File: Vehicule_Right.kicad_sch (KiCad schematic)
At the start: 16 parts, among them Q27 IRLZ44N, U7 LM339

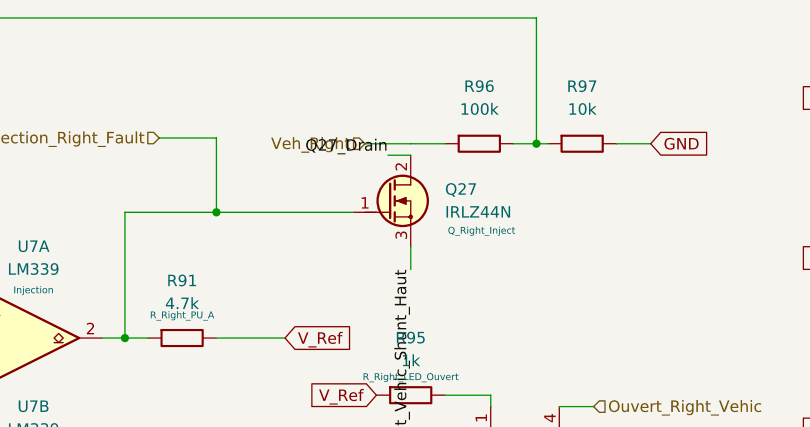
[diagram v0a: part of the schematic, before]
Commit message: Add files via upload
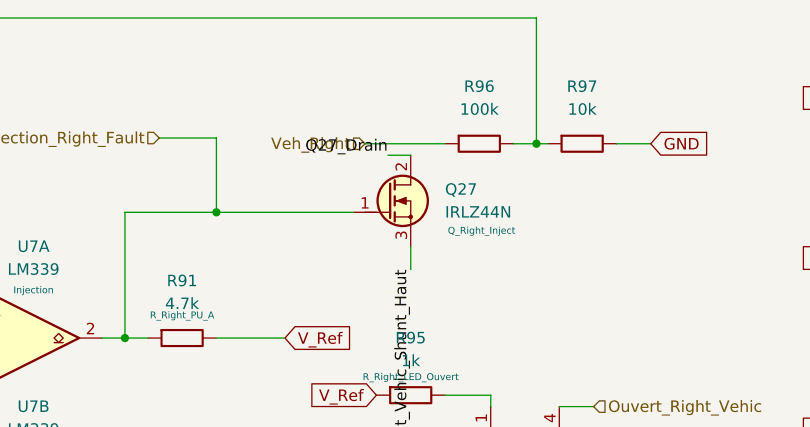
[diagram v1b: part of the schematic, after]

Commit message: Add files via upload
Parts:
- U7: footprint (none) -> Package_DIP:DIP-14_W7.62mm_Socket
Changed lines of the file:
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@@
 			)
 		)
-		(property "Footprint" ""
+		(property "Footprint" "Package_DIP:DIP-14_W7.62mm_Socket"
 			(at 110.49 134.62 0)
 			(hide yes)
@@
 			)
 		)
-		(property "Footprint" ""
+		(property "Footprint" "Package_DIP:DIP-14_W7.62mm_Socket"
 			(at 113.03 116.84 0)
 			(hide yes)
@@
 			)
 		)
-		(property "Footprint" ""
+		(property "Footprint" "Package_DIP:DIP-14_W7.62mm_Socket"
 			(at 113.03 85.09 0)
 			(hide yes)
@@
 			)
 		)
-		(property "Footprint" ""
+		(property "Footprint" "Package_DIP:DIP-14_W7.62mm_Socket"
 			(at 113.03 101.6 0)
 			(hide yes)
@@
 			)
 		)
-		(property "Footprint" ""
+		(property "Footprint" "Package_DIP:DIP-14_W7.62mm_Socket"
 			(at 113.03 67.31 0)
 			(hide yes)

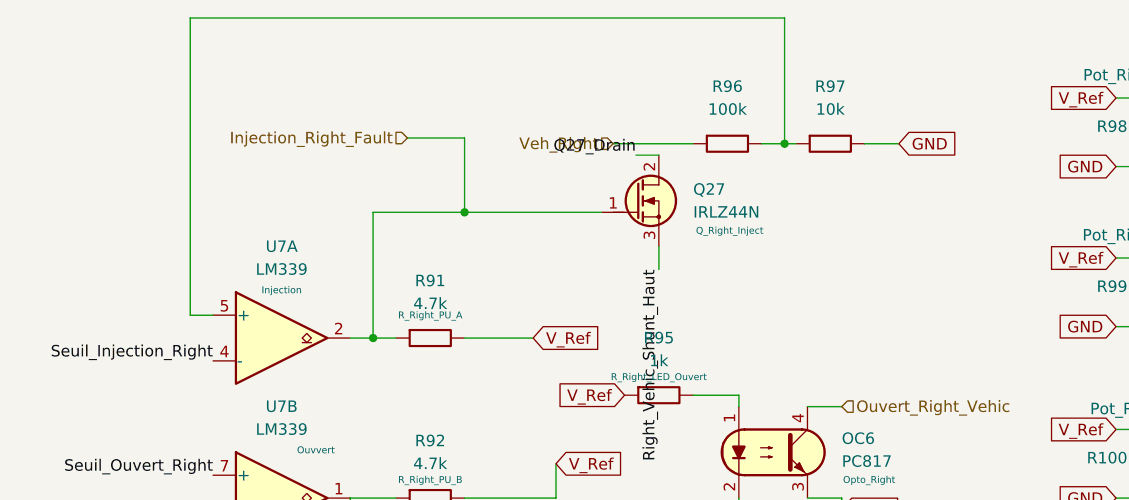
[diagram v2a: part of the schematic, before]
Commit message: Add files via upload
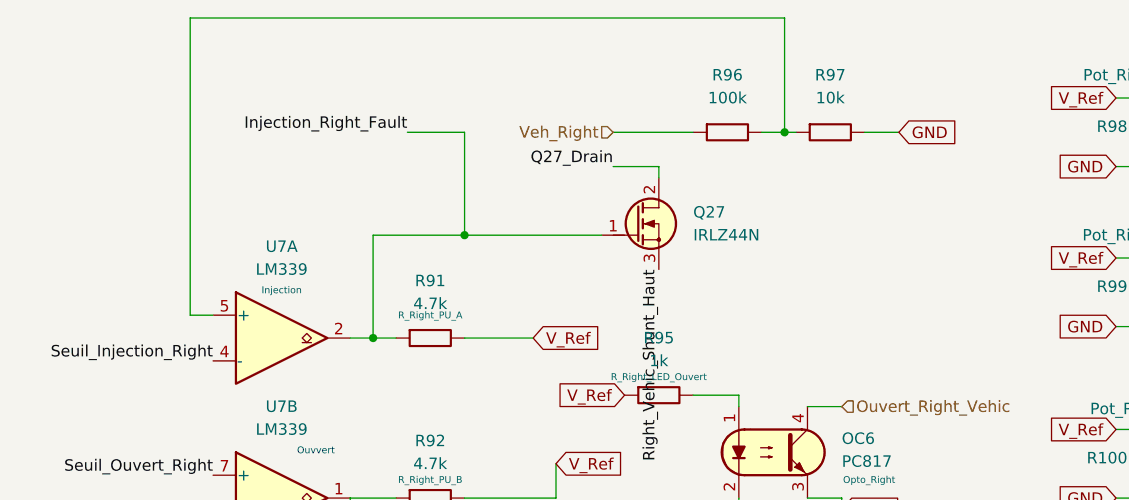
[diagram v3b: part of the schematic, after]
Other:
- moved on the sheet: Q27, R96, R97
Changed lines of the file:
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@@
 	)
 	(junction
-		(at 170.18 48.26)
+		(at 170.18 46.99)
 		(diameter 0)
 		(color 0 0 0 0)
 	)
 	(junction
-		(at 134.62 55.88)
+		(at 124.46 69.85)
 		(diameter 0)
 		(color 0 0 0 0)
 	)
 	(junction
-		(at 124.46 69.85)
+		(at 134.62 58.42)
 		(diameter 0)
 		(color 0 0 0 0)
@@
 	(wire
 		(pts
-			(xy 134.62 55.88) (xy 149.86 55.88)
+			(xy 134.62 58.42) (xy 149.86 58.42)
 		)
 		(stroke
@@
 	(wire
 		(pts
-			(xy 124.46 69.85) (xy 121.92 69.85)
+			(xy 156.21 50.8) (xy 156.21 52.07)
 		)
 		(stroke
@@
 	(wire
 		(pts
-			(xy 156.21 59.69) (xy 156.21 62.23)
+			(xy 124.46 69.85) (xy 121.92 69.85)
 		)
 		(stroke
@@
 	(wire
 		(pts
-			(xy 156.21 49.53) (xy 153.67 49.53)
-		)
-		(stroke
-			(width 0)
-			(type default)
-		)
-	)
-	(wire
-		(pts
 			(xy 207.01 68.58) (xy 210.82 68.58)
 		)
@@
 	(wire
 		(pts
-			(xy 170.18 48.26) (xy 170.18 34.29)
+			(xy 170.18 46.99) (xy 170.18 34.29)
 		)
 		(stroke
@@
 	(wire
 		(pts
-			(xy 170.18 48.26) (xy 171.45 48.26)
+			(xy 170.18 46.99) (xy 171.45 46.99)
 		)
 		(stroke
@@
 	(wire
 		(pts
-			(xy 179.07 48.26) (xy 182.88 48.26)
+			(xy 179.07 46.99) (xy 182.88 46.99)
 		)
 		(stroke
@@
 	(wire
 		(pts
-			(xy 134.62 47.625) (xy 134.62 55.88)
+			(xy 207.01 87.63) (xy 210.82 87.63)
 		)
 		(stroke
@@
 	(wire
 		(pts
-			(xy 207.01 87.63) (xy 210.82 87.63)
+			(xy 170.18 34.29) (xy 104.14 34.29)
 		)
 		(stroke
@@
 	(wire
 		(pts
-			(xy 170.18 34.29) (xy 104.14 34.29)
+			(xy 124.46 58.42) (xy 134.62 58.42)
 		)
 		(stroke
@@
 	(wire
 		(pts
-			(xy 124.46 55.88) (xy 134.62 55.88)
+			(xy 82.55 90.17) (xy 82.55 101.6)
 		)
 		(stroke
@@
 	(wire
 		(pts
-			(xy 82.55 90.17) (xy 82.55 101.6)
+			(xy 140.97 104.14) (xy 140.97 109.22)
 		)
 		(stroke
@@
 	(wire
 		(pts
-			(xy 140.97 104.14) (xy 140.97 109.22)
+			(xy 69.85 132.08) (xy 67.31 132.08)
 		)
 		(stroke
@@
 	(wire
 		(pts
-			(xy 69.85 132.08) (xy 67.31 132.08)
+			(xy 207.01 43.18) (xy 210.82 43.18)
 		)
 		(stroke
@@
 	(wire
 		(pts
-			(xy 207.01 43.18) (xy 210.82 43.18)
+			(xy 134.62 46.99) (xy 134.62 58.42)
 		)
 		(stroke
@@
 	(wire
 		(pts
-			(xy 151.13 48.26) (xy 160.02 48.26)
+			(xy 151.13 46.99) (xy 160.02 46.99)
 		)
 		(stroke
@@
 	(wire
 		(pts
-			(xy 128.27 47.625) (xy 134.62 47.625)
+			(xy 128.27 46.99) (xy 134.62 46.99)
 		)
 		(stroke
@@
 	(wire
 		(pts
-			(xy 167.64 48.26) (xy 170.18 48.26)
+			(xy 167.64 46.99) (xy 170.18 46.99)
 		)
 		(stroke
@@
 	(wire
 		(pts
-			(xy 124.46 55.88) (xy 124.46 69.85)
+			(xy 124.46 58.42) (xy 124.46 69.85)
 		)
 		(stroke
@@
 	(wire
 		(pts
+			(xy 151.13 50.8) (xy 156.21 50.8)
+		)
+		(stroke
+			(width 0)
+			(type default)
+		)
+	)
+	(wire
+		(pts
 			(xy 127 69.85) (xy 124.46 69.85)
 		)
@@
 		)
 	)
+	(label "Injection_Right_Fault"
+		(at 128.27 46.99 180)
+		(effects
+			(font
+				(size 1.27 1.27)
+			)
+			(justify right bottom)
+		)
+	)
 	(label "Seuil_Court_Right"
 		(at 214.63 83.82 0)
@@
 	)
 	(label "Q27_Drain"
-		(at 153.67 49.53 180)
+		(at 151.13 50.8 180)
 		(effects
 			(font
@@
 	(global_label "GND"
 		(shape input)
-		(at 182.88 48.26 0)
+		(at 182.88 46.99 0)
 		(fields_autoplaced yes)
 		(effects
@@
 		)
 		(property "Intersheetrefs" "${INTERSHEET_REFS}"
-			(at 189.7357 48.26 0)
+			(at 189.7357 46.99 0)
 			(hide yes)
 			(show_name no)
@@
 		)
 	)
-	(hierarchical_label "Injection_Right_Fault"
-		(shape input)
-		(at 128.27 47.625 180)
-		(effects
-			(font
-				(size 1.27 1.27)
-			)
-			(justify right)
-		)
-	)
 	(hierarchical_label "Veh_Right"
 		(shape input)
-		(at 151.13 48.26 180)
+		(at 151.13 46.99 180)
 		(effects
 			(font
@@
 	(symbol
 		(lib_id "PCM_SL_Resistors:100k")
-		(at 163.83 48.26 0)
+		(at 163.83 46.99 0)
 		(unit 1)
 		(body_style 1)
@@
 		(fields_autoplaced yes)
 		(property "Reference" "R96"
-			(at 163.83 41.91 0)
+			(at 163.83 40.64 0)
 			(show_name no)
 			(do_not_autoplace no)
@@
 		)
 		(property "Value" "100k"
-			(at 163.83 44.45 0)
+			(at 163.83 43.18 0)
 			(show_name no)
 			(do_not_autoplace no)
@@
 		)
 		(property "Footprint" "Resistor_THT:R_Axial_DIN0207_L6.3mm_D2.5mm_P10.16mm_Horizontal"
-			(at 164.719 52.578 0)
+			(at 164.719 51.308 0)
 			(hide yes)
 			(show_name no)
@@
 		)
 		(property "Datasheet" ""
-			(at 164.338 48.26 0)
+			(at 164.338 46.99 0)
 			(hide yes)
 			(show_name no)
@@
 		)
 		(property "Description" "100kΩ, 1/4W Resistor"
-			(at 163.83 48.26 0)
+			(at 163.83 46.99 0)
 			(hide yes)
 			(show_name no)
@@
 	(symbol
 		(lib_id "PCM_SL_Resistors:10k")
-		(at 175.26 48.26 0)
+		(at 175.26 46.99 0)
 		(unit 1)
 		(body_style 1)
@@
 		(fields_autoplaced yes)
 		(property "Reference" "R97"
-			(at 175.26 41.91 0)
+			(at 175.26 40.64 0)
 			(show_name no)
 			(do_not_autoplace no)
@@
 		)
 		(property "Value" "10k"
-			(at 175.26 44.45 0)
+			(at 175.26 43.18 0)
 			(show_name no)
 			(do_not_autoplace no)
@@
 		)
 		(property "Footprint" "Resistor_THT:R_Axial_DIN0207_L6.3mm_D2.5mm_P10.16mm_Horizontal"
-			(at 176.149 52.578 0)
+			(at 176.149 51.308 0)
 			(hide yes)
 			(show_name no)
@@
 		)
 		(property "Datasheet" ""
-			(at 175.768 48.26 0)
+			(at 175.768 46.99 0)
 			(hide yes)
 			(show_name no)
@@
 		)
 		(property "Description" "10kΩ, 1/4W Resistor"
-			(at 175.26 48.26 0)
+			(at 175.26 46.99 0)
 			(hide yes)
 			(show_name no)
@@
 	(symbol
 		(lib_id "PCM_Transistor_MOSFET_AKL:IRLZ44N")
-		(at 153.67 54.61 0)
+		(at 153.67 57.15 0)
 		(unit 1)
 		(body_style 1)
@@
 		(dnp no)
 		(property "Reference" "Q27"
-			(at 160.02 53.3399 0)
+			(at 160.02 55.8799 0)
 			(show_name no)
 			(do_not_autoplace no)
@@
 		)
 		(property "Value" "IRLZ44N"
-			(at 160.02 55.8799 0)
+			(at 160.02 58.4199 0)
 			(show_name no)
 			(do_not_autoplace no)
@@
 		)
 		(property "Footprint" "PCM_Package_TO_SOT_THT_AKL:TO-220-3_Vertical_GDS"
-			(at 158.75 52.07 0)
+			(at 158.75 54.61 0)
 			(hide yes)
 			(show_name no)
@@
 		)
 		(property "Datasheet" "https://www.tme.eu/Document/71cf1899624764088671ce6de5d15eb4/irlz44n.pdf"
-			(at 153.67 54.61 0)
+			(at 153.67 57.15 0)
 			(hide yes)
 			(show_name no)
@@
 		)
 		(property "Description" "TO-220 N-MOSFET enchancement mode transistor, 55V, 47A, 110W, Alternate KiCAD Library"
-			(at 153.67 54.61 0)
+			(at 153.67 57.15 0)
 			(hide yes)
 			(show_name no)
@@
 		)
 		(property "Etiquette" "Q_Right_Inject"
-			(at 164.084 57.912 0)
+			(at 164.084 60.452 0)
+			(hide yes)
 			(show_name no)
 			(do_not_autoplace no)
